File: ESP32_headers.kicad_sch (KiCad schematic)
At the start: 2 parts, among them J1 Conn_01x15_Socket, J2 Conn_01x15_Socket

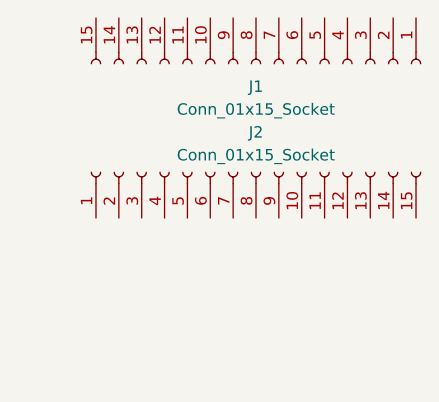
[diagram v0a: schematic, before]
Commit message: merge labels
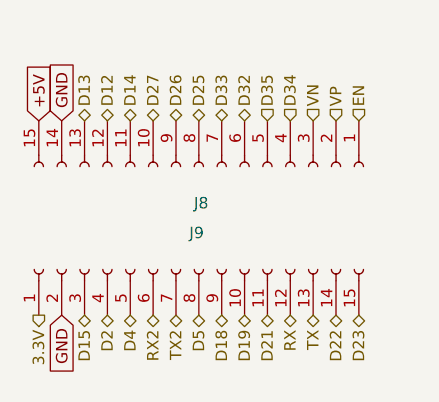
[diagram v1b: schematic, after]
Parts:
- removed J1, J2: Conn_01x15_Socket, Connector_PinSocket_2.54mm:PinSocket_1x15_P2.54mm_Vertical, symbol Connector:Conn_01x15_Socket
- added J8, J9: Conn_01x15_Socket, Connector_PinSocket_2.54mm:PinSocket_1x15_P2.54mm_Vertical, symbol Connector:Conn_01x15_Socket
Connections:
- new net +5V: J8.15 (Pin_15)
- new net 3.3V: J9.1 (Pin_1)
- new net D12: J8.12 (Pin_12)
- new net D13: J8.13 (Pin_13)
- new net D14: J8.11 (Pin_11)
- new net D15: J9.3 (Pin_3)
- new net D18: J9.9 (Pin_9)
- new net D19: J9.10 (Pin_10)
- new net D2: J9.4 (Pin_4)
- new net D21: J9.11 (Pin_11)
- new net D22: J9.14 (Pin_14)
- new net D23: J9.15 (Pin_15)
- new net D25: J8.8 (Pin_8)
- new net D26: J8.9 (Pin_9)
- new net D27: J8.10 (Pin_10)
- new net D32: J8.6 (Pin_6)
- new net D33: J8.7 (Pin_7)
- new net D34: J8.4 (Pin_4)
- new net D35: J8.5 (Pin_5)
- new net D4: J9.5 (Pin_5)
- new net D5: J9.8 (Pin_8)
- new net EN: J8.1 (Pin_1)
- new net GND: J8.14 (Pin_14), J9.2 (Pin_2)
- new net RX: J9.12 (Pin_12)
- new net RX2: J9.6 (Pin_6)
- new net TX: J9.13 (Pin_13)
- new net TX2: J9.7 (Pin_7)
- new net VN: J8.3 (Pin_3)
- new net VP: J8.2 (Pin_2)
